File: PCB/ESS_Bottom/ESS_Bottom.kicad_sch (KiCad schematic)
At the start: 14 parts, among them J10 Conn_01x01, J11 Conn_01x01, J12 Conn_01x01, J5 Conn_01x01, J6 Conn_01x01, J7 Conn_01x01, J8 Conn_01x01, J9 Conn_01x01, SW1 SW_Slide_DPDT, U3 ESP32-C3-DevKitM-1

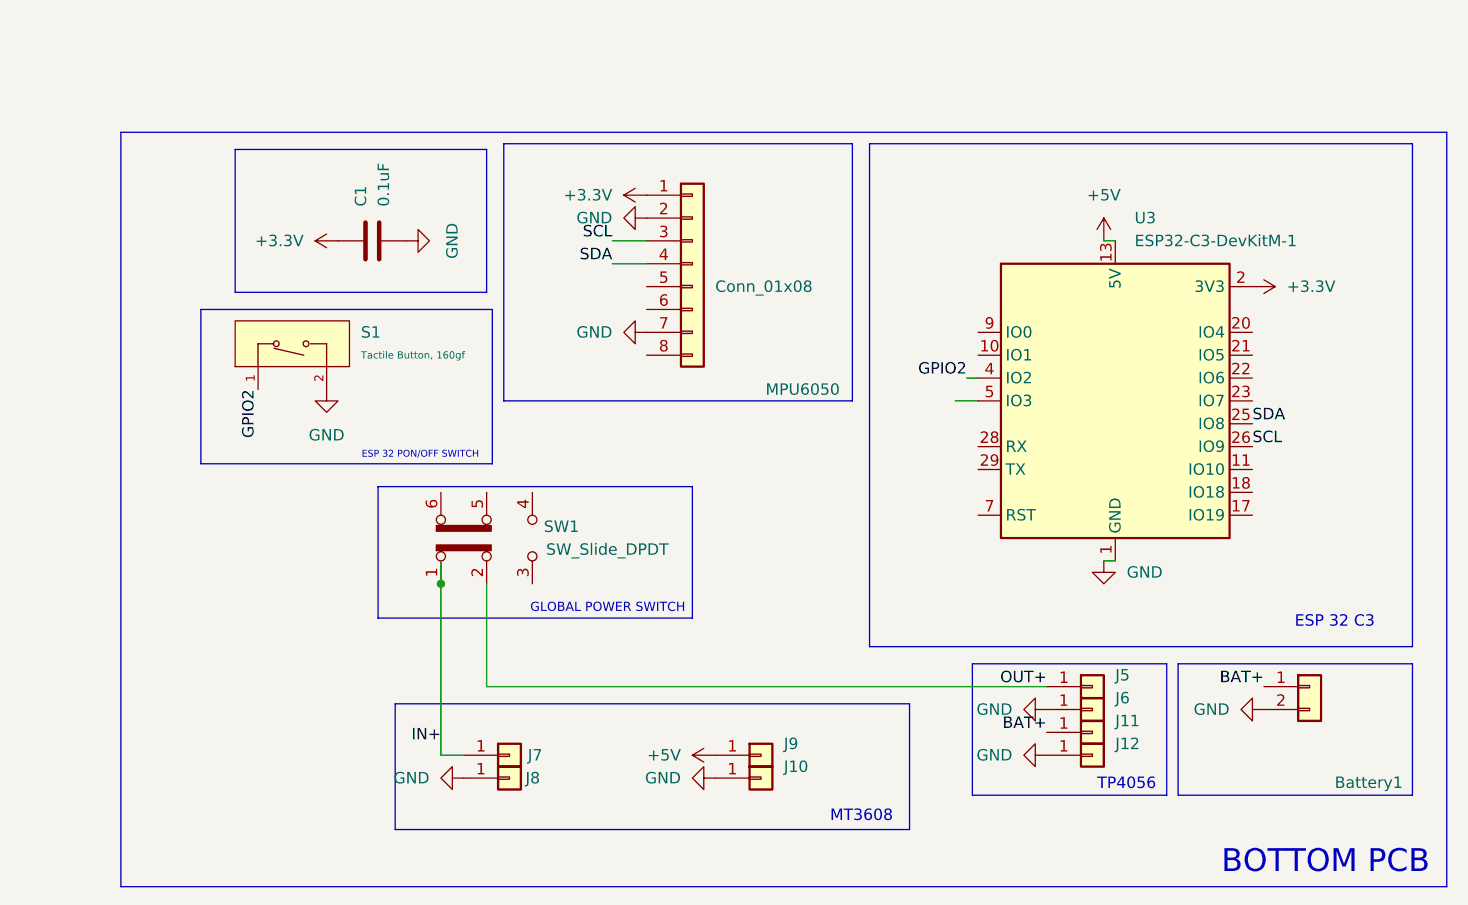
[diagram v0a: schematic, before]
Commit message: made kicad files cleaner?
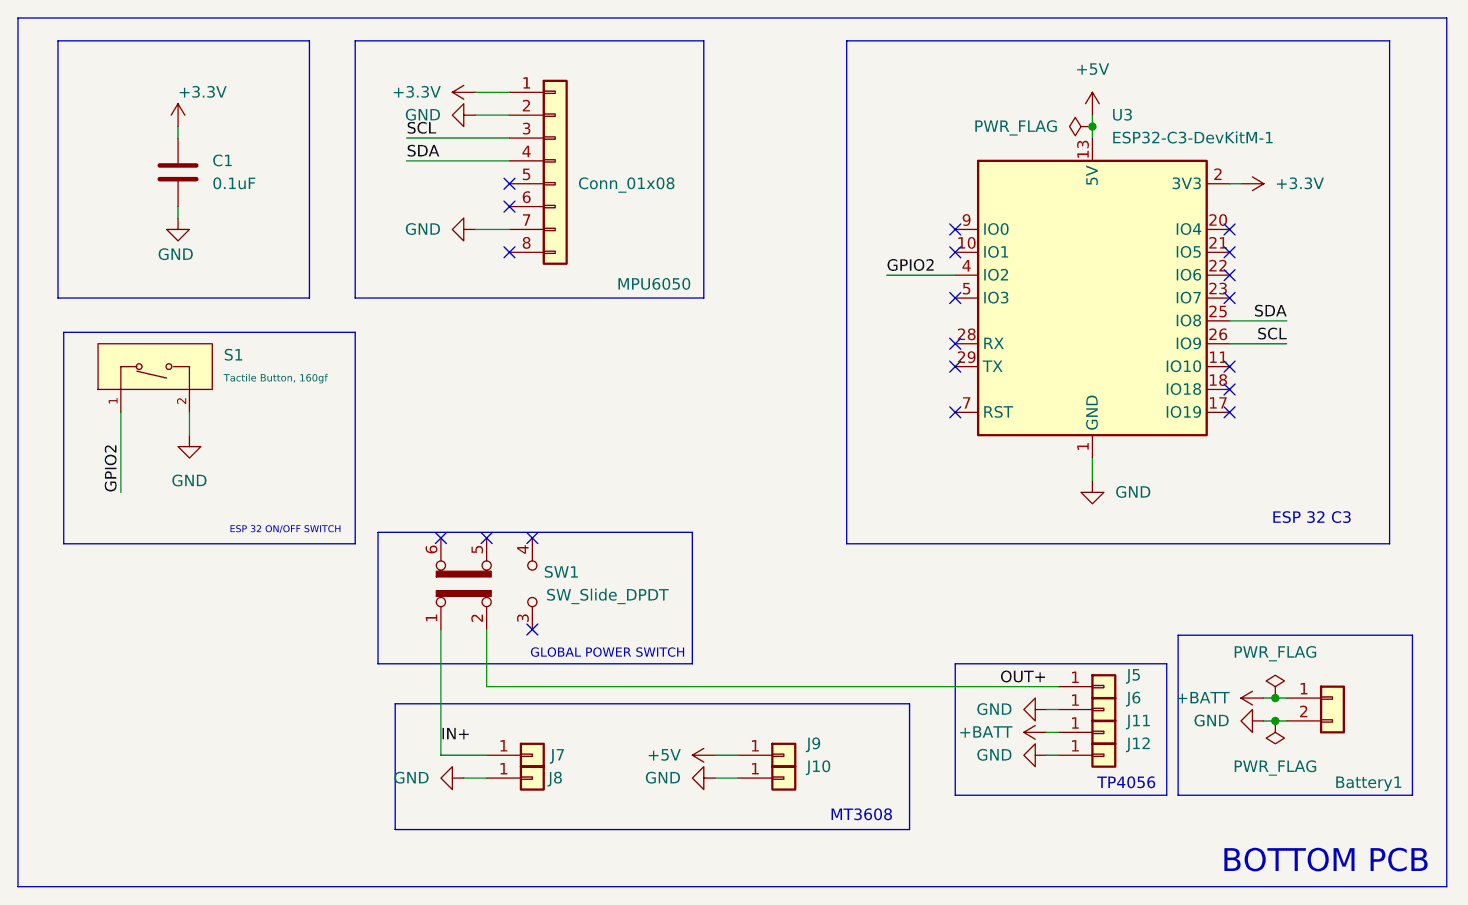
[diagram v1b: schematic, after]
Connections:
- net BAT+ renamed +BATT
- no-connect marks 0 -> 20
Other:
- note added: "ESP 32 ON/OFF SWITCH"
- note removed: "ESP 32 PON/OFF SWITCH"
- moved on the sheet: Battery1, C1, J10, J11, J12, J5, J6, J7, J8, J9, MPU6050, S1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
